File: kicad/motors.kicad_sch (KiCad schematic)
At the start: 73 parts, among them J12 Conn_01x04_Pin, J3 Conn_01x04_Pin, J4 Conn_01x04_Pin, J5 Conn_01x04_Pin, J6 Conn_01x04_Pin, U2 TB67S109AFTG, U3 TB67S109AFTG, U4 TB67S109AFTG, U6 TB67S109AFTG

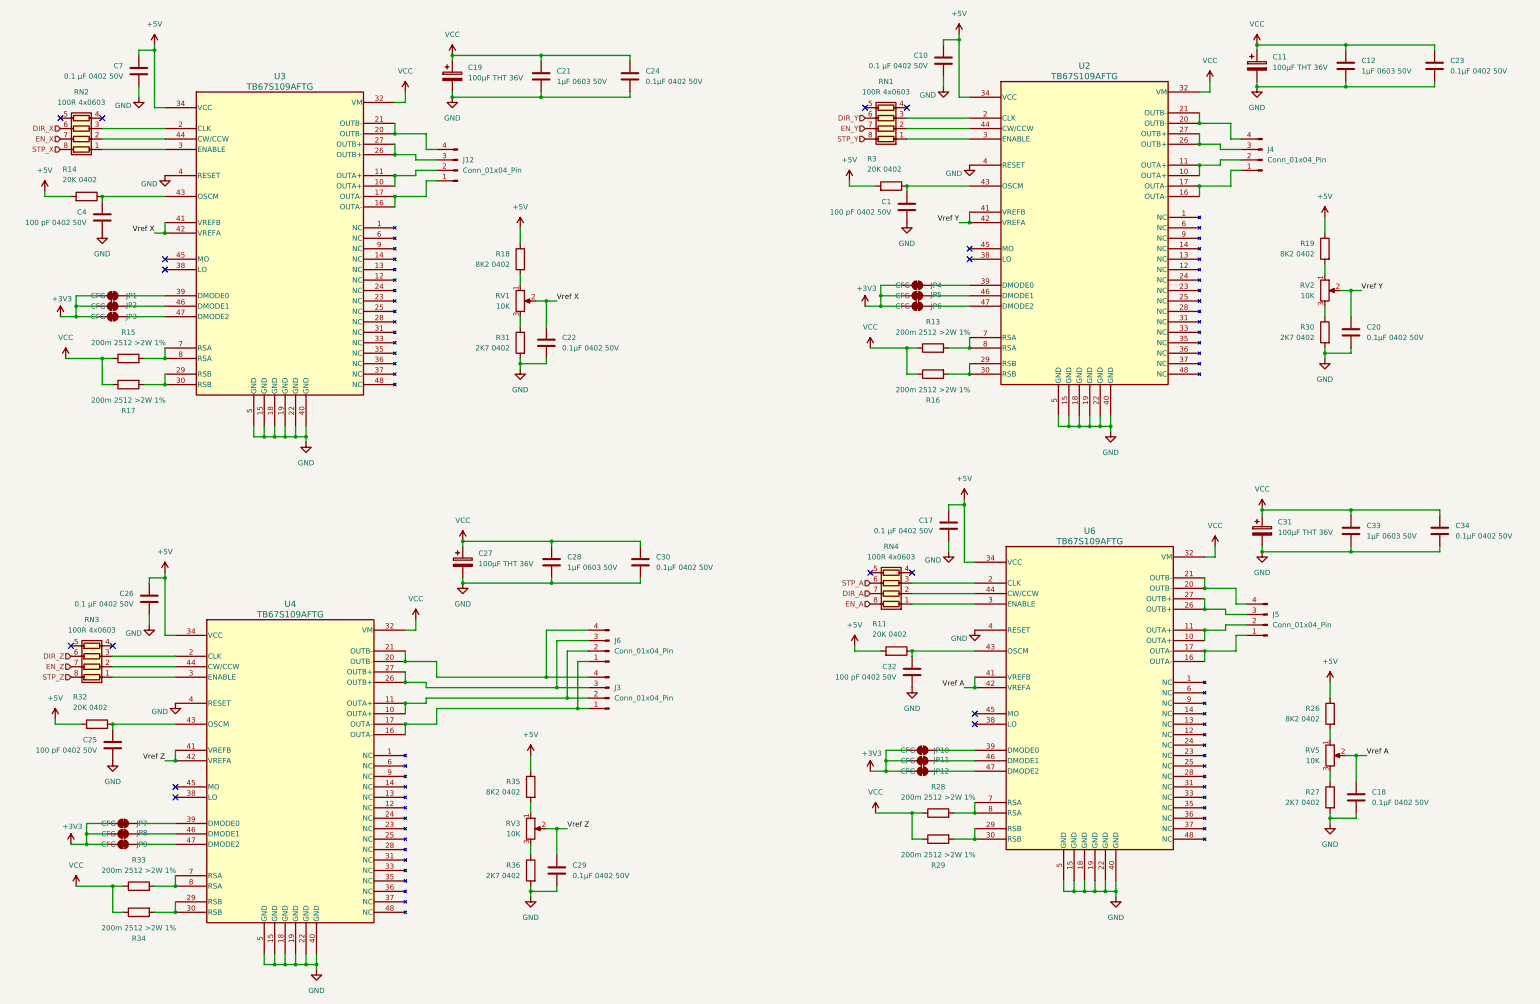
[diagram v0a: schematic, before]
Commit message: layout progress
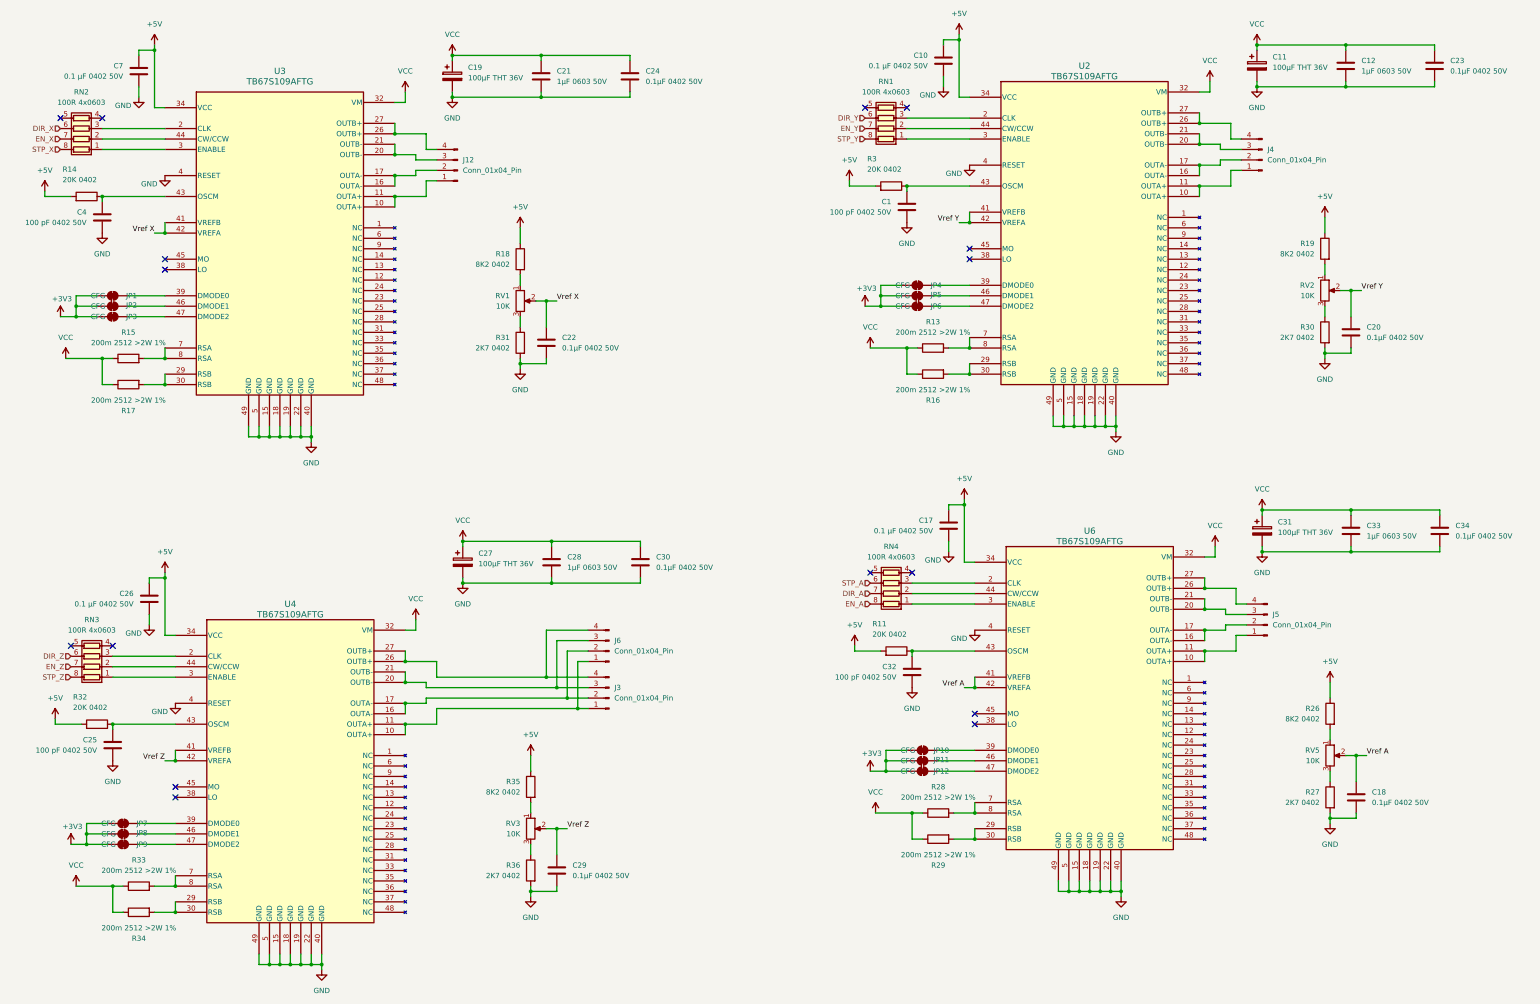
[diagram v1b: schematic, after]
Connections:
- net GND: now also U2.49 (GND), U3.49 (GND), U4.49 (GND), U6.49 (GND)
- net at U4.10 (OUTA+), U4.11 (OUTA+): now also J3.1 (Pin_1), J6.1 (Pin_1); no longer J3.2 (Pin_2), J6.2 (Pin_2)
- net at U4.16 (OUTA-), U4.17 (OUTA-): now also J3.2 (Pin_2), J6.2 (Pin_2); no longer J3.1 (Pin_1), J6.1 (Pin_1)
- net at U4.20 (OUTB-), U4.21 (OUTB-): now also J3.3 (Pin_3), J6.3 (Pin_3); no longer J3.4 (Pin_4), J6.4 (Pin_4)
- net at U4.26 (OUTB+), U4.27 (OUTB+): now also J3.4 (Pin_4), J6.4 (Pin_4); no longer J3.3 (Pin_3), J6.3 (Pin_3)
- net at U3.16 (OUTA-), U3.17 (OUTA-): now also J12.2 (Pin_2); no longer J12.1 (Pin_1)
- net at U3.10 (OUTA+), U3.11 (OUTA+): now also J12.1 (Pin_1); no longer J12.2 (Pin_2)
- net at U3.26 (OUTB+), U3.27 (OUTB+): now also J12.4 (Pin_4); no longer J12.3 (Pin_3)
- net at U3.20 (OUTB-), U3.21 (OUTB-): now also J12.3 (Pin_3); no longer J12.4 (Pin_4)
- net at U6.10 (OUTA+), U6.11 (OUTA+): now also J5.1 (Pin_1); no longer J5.2 (Pin_2)
- net at U6.16 (OUTA-), U6.17 (OUTA-): now also J5.2 (Pin_2); no longer J5.1 (Pin_1)
- net at U6.20 (OUTB-), U6.21 (OUTB-): now also J5.3 (Pin_3); no longer J5.4 (Pin_4)
- net at U6.26 (OUTB+), U6.27 (OUTB+): now also J5.4 (Pin_4); no longer J5.3 (Pin_3)
- net at U2.16 (OUTA-), U2.17 (OUTA-): now also J4.2 (Pin_2); no longer J4.1 (Pin_1)
- net at U2.10 (OUTA+), U2.11 (OUTA+): now also J4.1 (Pin_1); no longer J4.2 (Pin_2)
- net at U2.26 (OUTB+), U2.27 (OUTB+): now also J4.4 (Pin_4); no longer J4.3 (Pin_3)
- net at U2.20 (OUTB-), U2.21 (OUTB-): now also J4.3 (Pin_3); no longer J4.4 (Pin_4)
